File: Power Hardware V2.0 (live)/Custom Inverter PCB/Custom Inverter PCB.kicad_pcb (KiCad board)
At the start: 2 copper layers, 173 x 148 mm, 86 parts, among them J1 1714971, J2 1714971, J3 1714968, J6 1989764, J7 1714971, J8 1714971, K2 1-1393210-3, Q1 CSD19532Q5B, Q2 CSD19532Q5B, Q3 CSD19532Q5B, Q4 CSD19532Q5B, Q5 CSD19532Q5B, Q6 CSD19532Q5B, U1 DRV8300DIPWR, U2 TLI4971A050T5E0001XUMA1, U3 TLI4971A050T5E0001XUMA1, U4 TLI4971A050T5E0001XUMA1, U5 LAUNCHXL-F280049C, U6 OP292GSZ-REEL

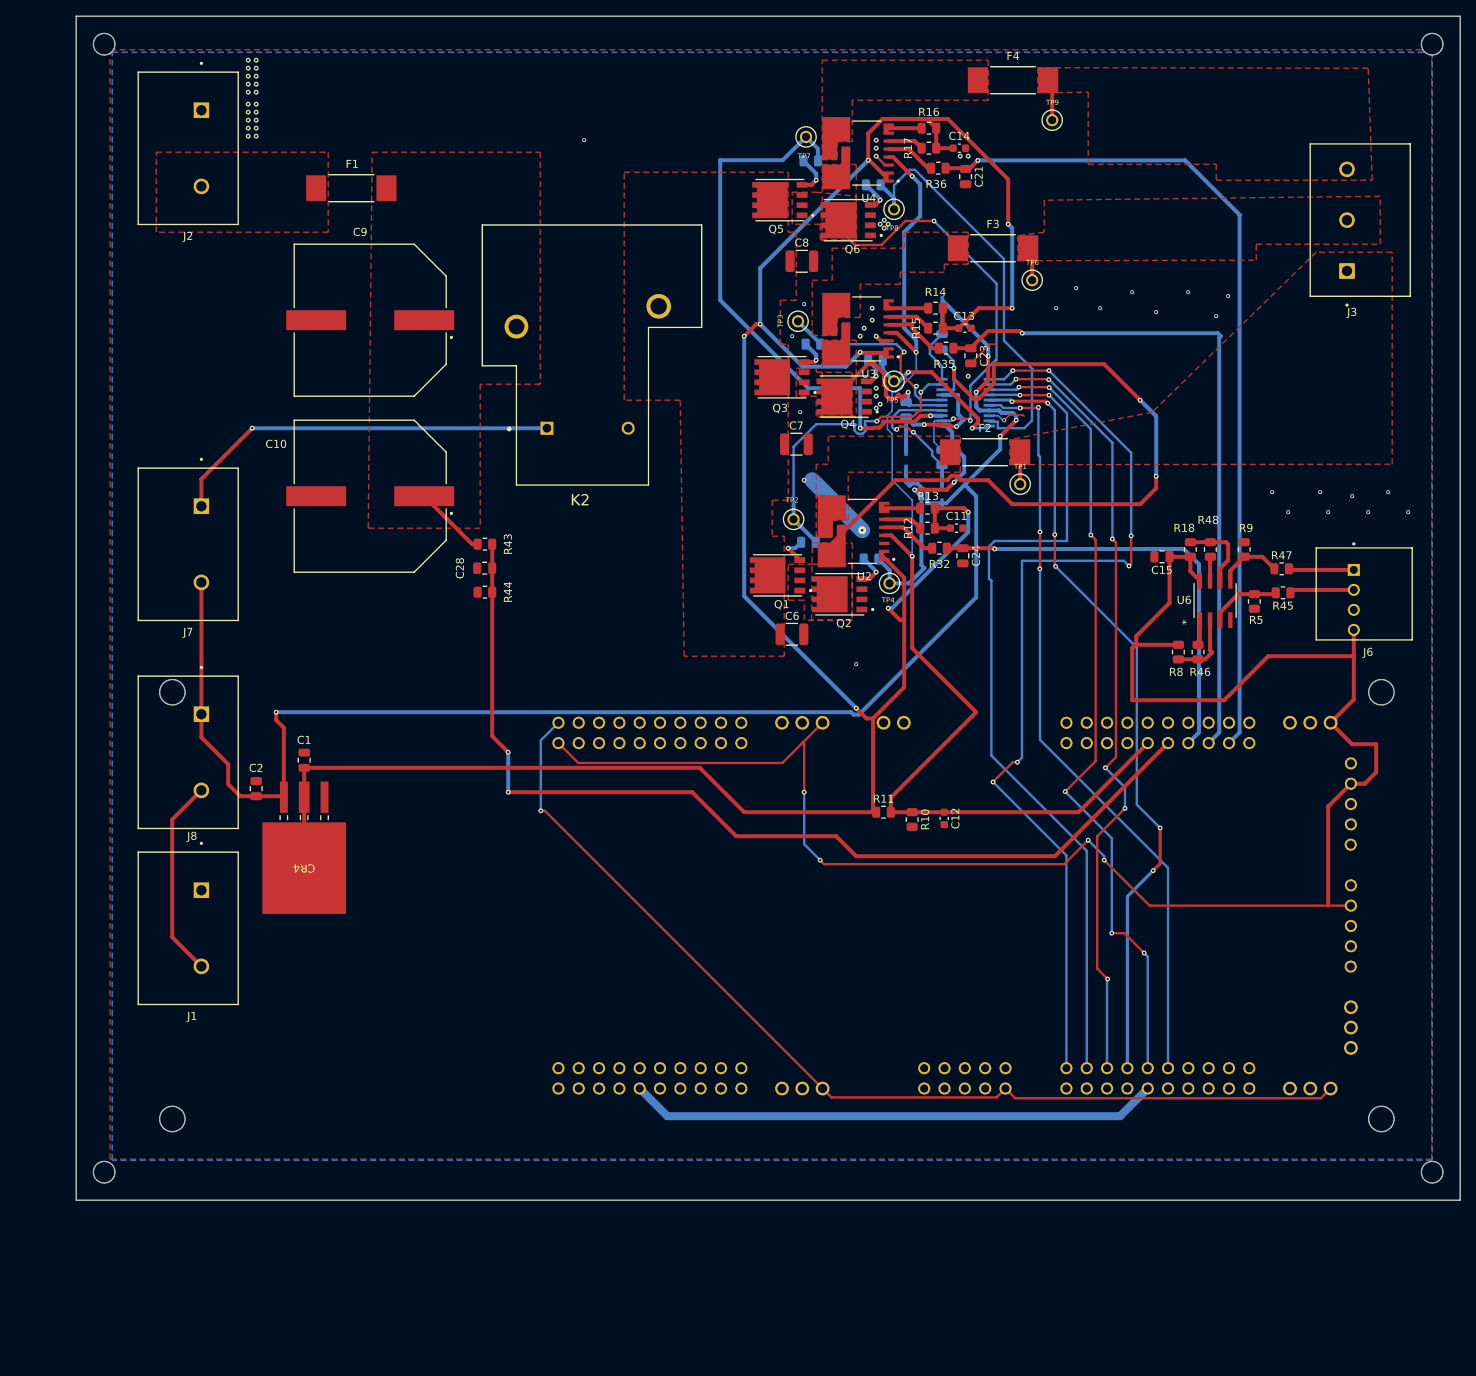
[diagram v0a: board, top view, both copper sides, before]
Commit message: PCB Fixes
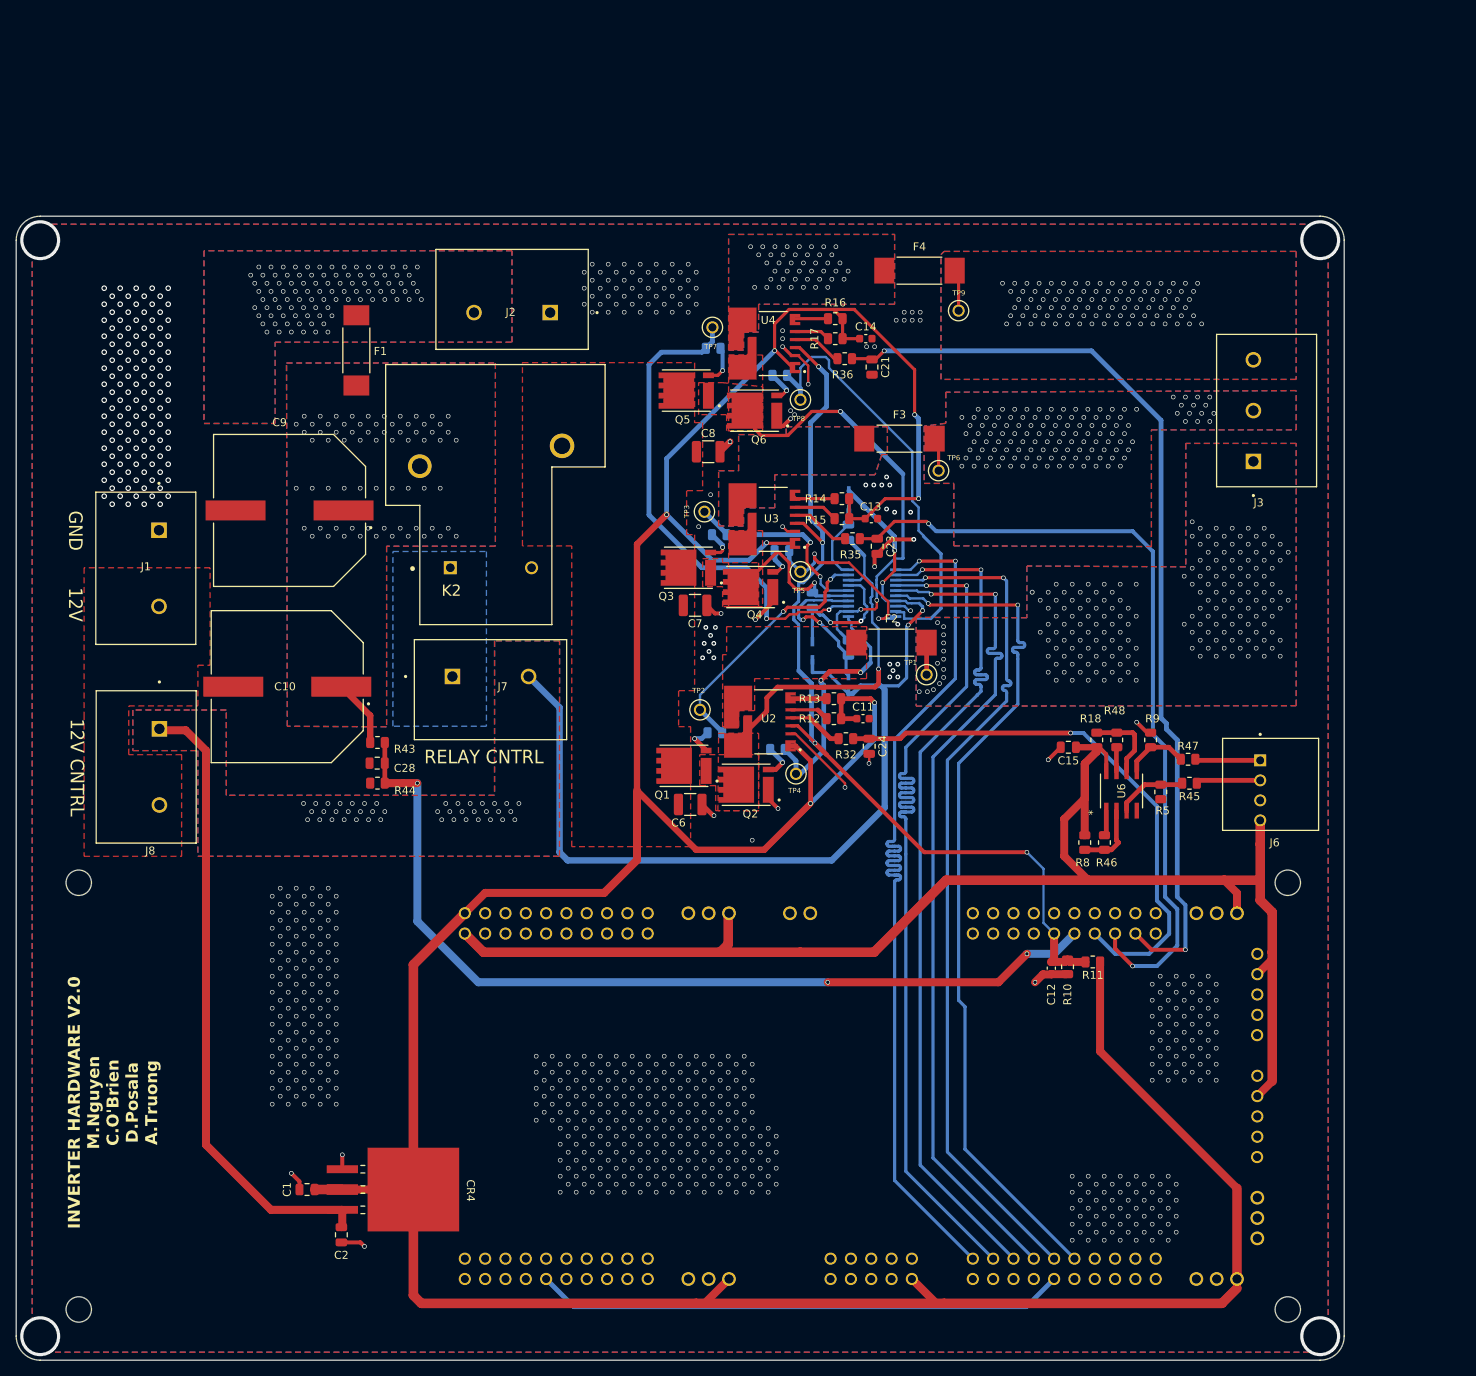
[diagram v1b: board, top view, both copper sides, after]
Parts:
- removed REF** (x4): MountingHole_2.7mm_M2.5, MountingHole:MountingHole_2.7mm_M2.5
- moved J2 60.5 mm to (103.5, 21.1), turned to 180 degrees
- moved C2 56.8 mm to (72.6, 144.3), turned to -90 degrees
- moved C1 53.7 mm to (68.4, 138.7), turned to 180 degrees
- moved J7 48.4 mm to (81.8, 82.4), turned to 0 degrees
- moved J1 45.3 mm to (42.0, 51.5)
- moved CR4 42.4 mm to (81.6, 138.7), turned to -90 degrees
- moved R11 32.2 mm to (166.6, 110.2), turned to 180 degrees
- moved R43 28.2 mm to (77.2, 82.8)
- moved C28 27.8 mm to (77.1, 85.4)
- moved R44 27.4 mm to (77.2, 87.9)
- moved R10 26.8 mm to (163.4, 110.8)
- moved C11 26.5 mm to (137.8, 79.8)
- moved C14 26.5 mm to (138.2, 32.3)
- moved R16 26.5 mm to (134.4, 29.8)
- moved R17 26.5 mm to (134.4, 32.3)
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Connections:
- net Net-(F1-Pad1) renamed /GateDriver&Power Inputs/PVDD
- C1 pad 1: +3.3VDC -> +3.3V
- C11 pad 2: +3.3VDC -> +3.3V
- C13 pad 2: +3.3VDC -> +3.3V
- C14 pad 2: +3.3VDC -> +3.3V
- CR4 pad 2: +3.3VDC -> +3.3V
- CR4 pad 4: +3.3VDC -> +3.3V
- R11 pad 1: +3.3VDC -> +3.3V
- R12 pad 1: +3.3VDC -> +3.3V
- R13 pad 1: +3.3VDC -> +3.3V
- R14 pad 1: +3.3VDC -> +3.3V
- R15 pad 1: +3.3VDC -> +3.3V
- R16 pad 1: +3.3VDC -> +3.3V
- R17 pad 1: +3.3VDC -> +3.3V
- U2 pad 1: +3.3VDC -> +3.3V
- U3 pad 1: +3.3VDC -> +3.3V
- U4 pad 1: +3.3VDC -> +3.3V
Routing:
- net +3.3V: track 127.0 -> 463.0 mm, vias 1 -> 7
- net +3.3VDC: track 314.3 -> 0.00 mm, vias 9 -> 0
- net /SHA: track 98.7 -> 45.8 mm, vias 3 -> 1
- net Net-(J7-Pad1): track 49.2 -> 0.00 mm, vias 1 -> 0
- net GND: track 22.3 -> 57.4 mm, vias 63 -> 740
- net +5V: track 227.7 -> 192.9 mm, vias 4 -> 0
- net +12V to relay: track 25.0 -> 0.00 mm
- net /Current sense/Vref: track 141.1 -> 116.1 mm, vias 3 -> 4
- net /Current sense/ISENB: track 86.1 -> 101.2 mm, vias 1 -> 2
- net /Current sense/ISENA: track 55.3 -> 70.0 mm
- net /INLC: track 95.6 -> 108.9 mm, vias 4 -> 2
- net +12VDC: track 198.7 -> 211.0 mm, vias 5 -> 46
- net /Current sense/ISENC: track 106.6 -> 117.2 mm, vias 1 -> 2
- net /SEN_100V: track 123.5 -> 114.2 mm, vias 2 -> 3
- net /INLB: track 98.2 -> 107.1 mm, vias 6 -> 2
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- added copper zone on B.Cu, net +100VDC to Relay
- added copper zone on F.Cu, net +12V to relay
- added copper zone on B.Cu, net +12VDC
- added copper zone on F.Cu, net +12VDC
- added copper zone on B.Cu, net /Current sense/IB-
- added copper zone on B.Cu, net /Current sense/IC-
- added copper zone on B.Cu, net /GateDriver&Power Inputs/PVDD
- added copper zone on B.Cu, net /MOTA
- added copper zone on B.Cu, net /MOTB
- added copper zone on B.Cu, net /MOTC
- added copper zone on B.Cu, net Net-(J7-Pad1)
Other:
- board size 173 x 148 mm -> 166 x 143 mm
- board text added: "12V"
- board text added: "12V CNTRL"
- board text added: "GND"
- board text added: "INVERTER HARDWARE V2.0 M.Nguyen C.O'Brien D.Posala A.Truong"
- board text added: "RELAY CNTRL"
